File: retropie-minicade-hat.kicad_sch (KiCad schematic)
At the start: 17 parts, among them J1 40HAT, J2 Screw_Terminal_01x02, J3 Conn_02x02_Odd_Even, J4 Conn_02x02_Odd_Even, J5 Conn_01x08_Male, J6 Conn_01x08_Male, J7 Conn_01x03_Male, J8 Conn_02x03_Odd_Even, Q1 DMG2305UX, Q2 MMDT5401, U1 AMS1117-3.3

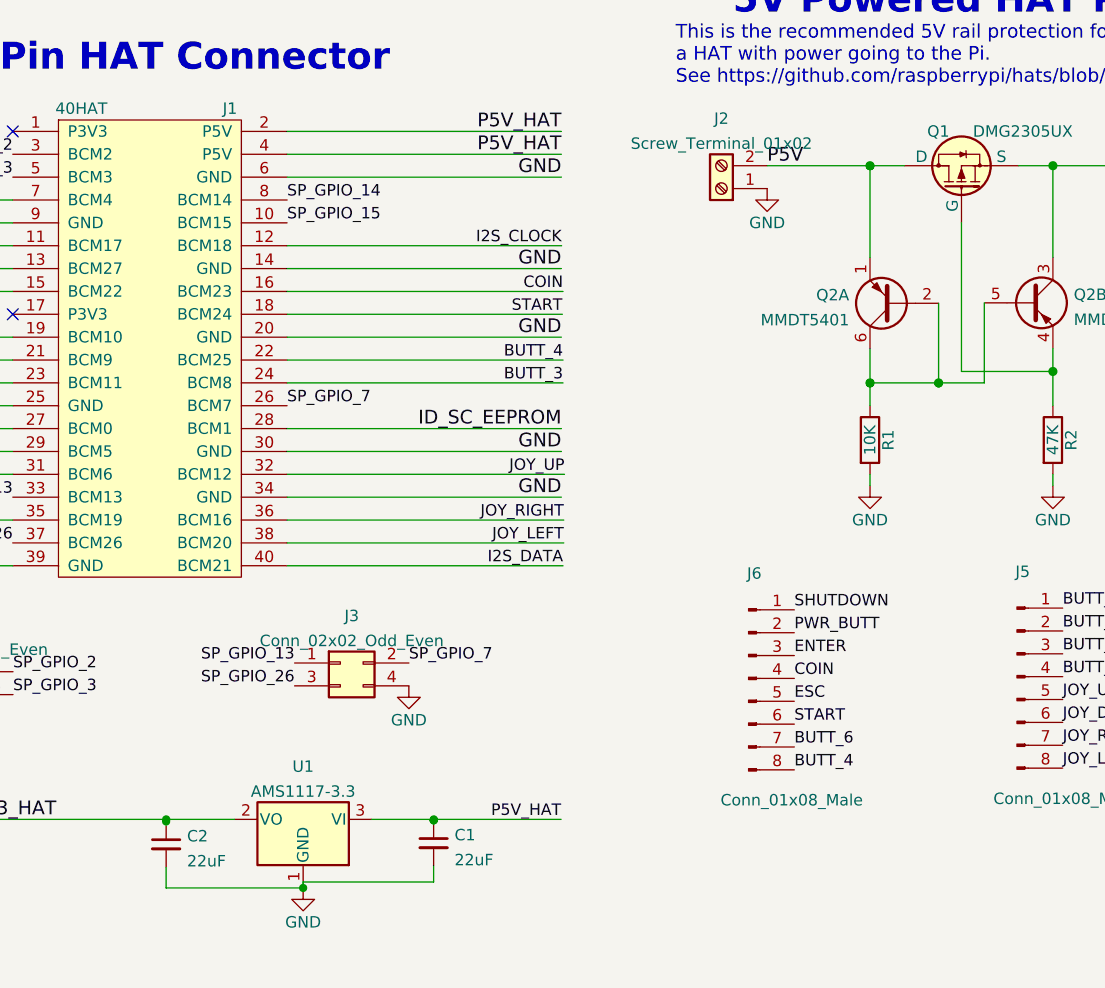
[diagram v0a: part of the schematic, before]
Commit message: updated images and gerbers (Rev2)
updated gerbers to latest version of PCB
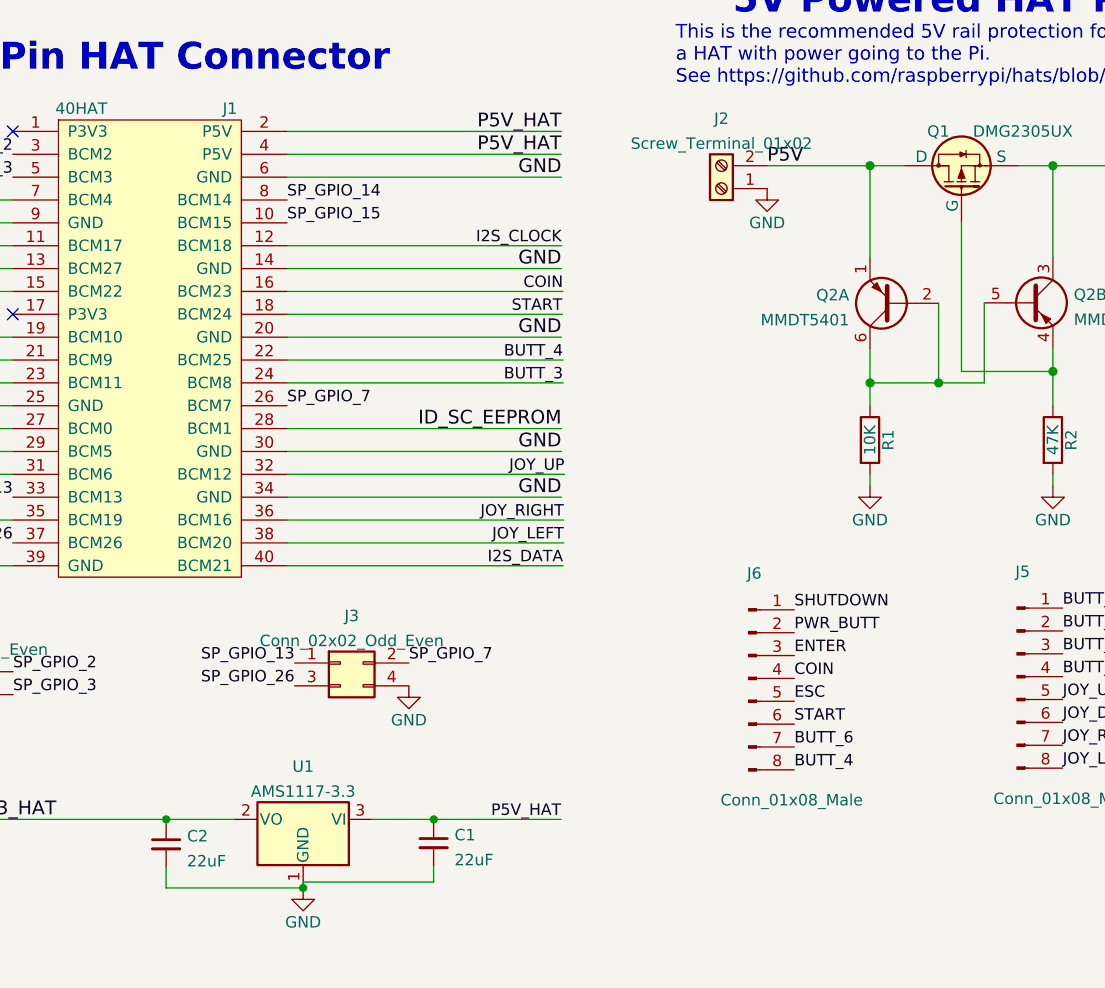
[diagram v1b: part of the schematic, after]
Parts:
- C1, C2: LCSC Part # C86295 -> C59461
- J2: footprint TerminalBlock:TerminalBlock_bornier-2_P5.08mm -> TerminalBlock_4Ucon:TerminalBlock_4Ucon_1x02_P3.50mm_Horizontal
- U1: LCSC Part # C173386 -> C6186
